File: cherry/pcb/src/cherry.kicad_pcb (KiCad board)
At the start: 4 copper layers, 61.2 x 26.1 mm, 73 parts, among them J1 USB4085-GF-A, J2 PinHeader_1x24, J3 PinHeader_1x24, J4 PinHeader_1x06, J5 PinHeader_1x06, J6 PinHeader_1x06, SW1 RESET, SW2 USER, U1 FT2232HL, U2 W25Q32JVSSIM, U3 ICE40LP8K-CM81, U4 TPS62A02, U5 TPS62A02, X1 ASE-12.000MHZ-LR-T

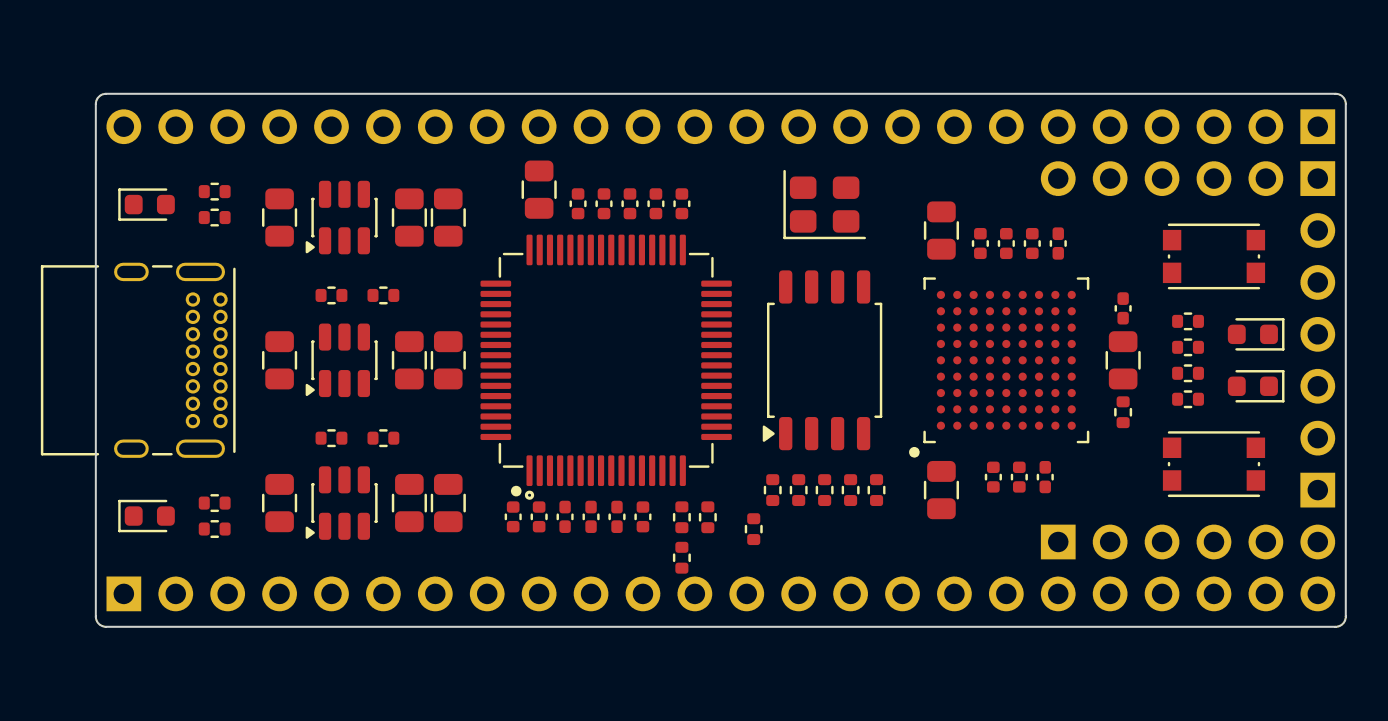
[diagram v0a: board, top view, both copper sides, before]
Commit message: wip
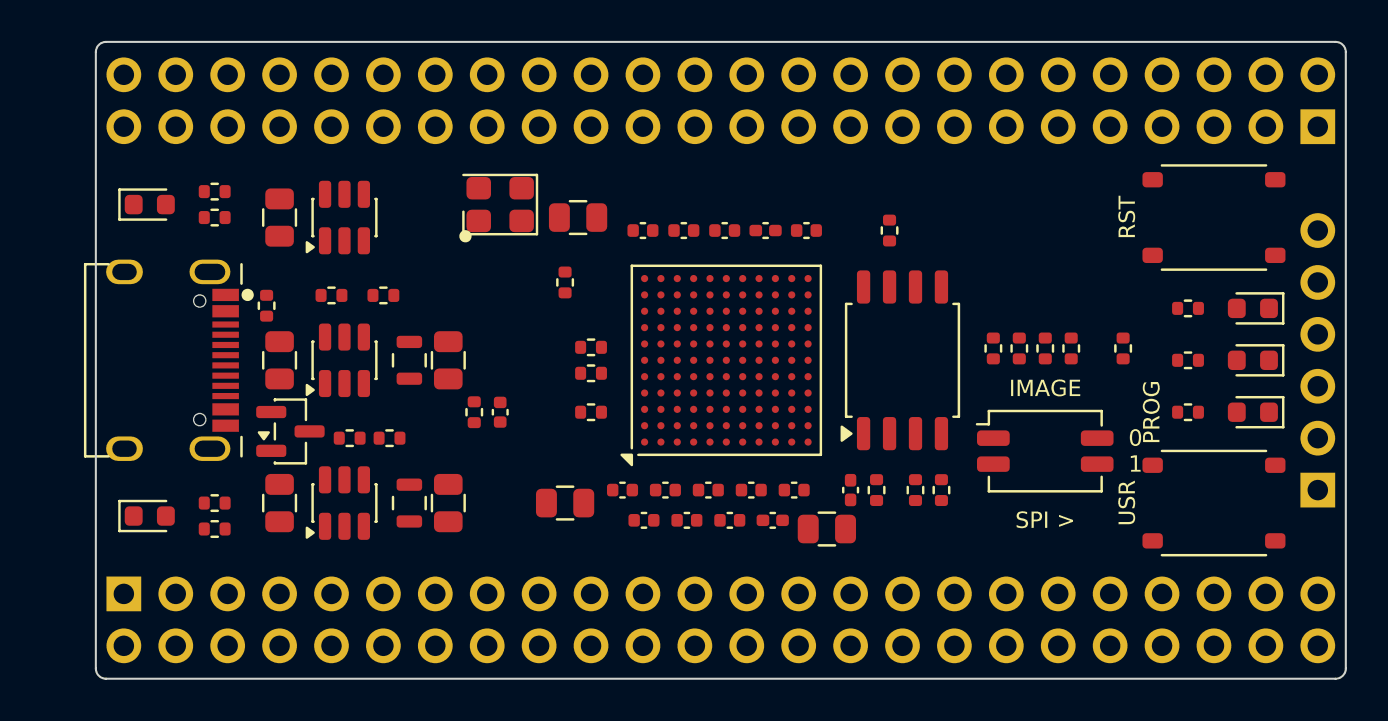
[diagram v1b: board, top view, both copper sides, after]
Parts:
- removed C12, C13, C14, C15: 100nF, Cherry:C_0402_1005Metric
- removed C26, C5: 10uF, Cherry:C_0805_2012Metric
- removed FB2: BLM21AG601SH1D, Cherry:L_0805_2012Metric
- removed J4, J6: PinHeader_1x06, Cherry:PinHeader_1x06_P2.54mm
- removed R18: 1k, Cherry:R_0402_1005Metric
- removed R7: 12k, Cherry:R_0402_1005Metric
- removed U1: FT2232HL, Cherry:LQFP-64_10x10mm_P0.5mm
- added C29: 100nF, Cherry:C_0402_1005Metric, F.Cu at (120.0, 92.7)
- added D6: LED_AMBER_0603, Cherry:LED_0603_1608Metric, F.Cu at (156.8, 92.7)
- added Q1: BSS138, Package_TO_SOT_SMD:SOT-23, F.Cu at (109.8, 93.7)
- added R23: 10k, Cherry:R_0402_1005Metric, F.Cu at (146.7, 89.6)
- added R24: 10k, Cherry:R_0402_1005Metric, F.Cu at (148.0, 89.6)
- added R25: 1k, Cherry:R_0402_1005Metric, F.Cu at (144.1, 89.6)
- added R26: 1k, Cherry:R_0402_1005Metric, F.Cu at (145.4, 89.6)
- added R27: 10k, Cherry:R_0402_1005Metric, F.Cu at (150.5, 89.6)
- added R29: 1k, Cherry:R_0402_1005Metric, F.Cu at (153.7, 92.7)
- added SW3: USER, Cherry:SW_Tactile_XKB_TS-1187A, F.Cu at (154.9, 97.2)
- D1: value PWR -> KT-0603R
- D2: value CFG -> KT-0603R
- D3: value USER0 -> KT-0603R
- D4: value USER1 -> KT-0603R
- FB1: value BLM21AG601SH1D -> GZ2012D601TF
- J1: value USB4085-GF-A -> TYPE-C-31-M-12; footprint Cherry:USB_C_Receptacle_GCT_USB4085 -> Cherry:USB_C_Receptacle_Hroparts_TYPE-C-31-M-12
- J2, J3: value PinHeader_1x24 -> PinHeader_2x24_Duplicate; footprint Cherry:PinHeader_1x24_P2.54mm -> Cherry:PinHeader_2x24_P2.54mm_Duplicate
- J5: value PinHeader_1x06 -> SPI PROGRAM
- L1, L2: value 1uH -> TFM201208ALD-1R0MTCA; footprint Cherry:L_0805_2012Metric -> Cherry:L_TDK_TFM201208ALD
- R14, R15: value 470 -> 68
- R16: value 470 -> 1.5k
- R17: value 470 -> 10k
- R9: value 10k -> 100k
- SW1: value RESET -> TS-1187A-B-A-B; footprint Cherry:SW_Push_1P1T_NO_CK_KMR2 -> Cherry:SW_Tactile_XKB_TS-1187A
- SW2: value USER -> IMAGE SELECT; footprint Cherry:SW_Push_1P1T_NO_CK_KMR2 -> Button_Switch_SMD:SW_DIP_SPSTx02_Slide_Copal_CHS-02A_W5.08mm_P1.27mm_JPin
- U2: value W25Q32JVSSIM -> W25Q32JVSSIQ
- U3: value ICE40LP8K-CM81 -> ICE40HX8K-BG121; footprint Cherry:BGA-81_9x9_8.0x8.0mm_P0.8mm -> Package_BGA:BGA-121_9.0x9.0mm_Layout11x11_P0.8mm_Ball0.4mm_Pad0.35mm_NSMD
- U4, U5: value TPS62A02 -> TPS62A02APDDCR
- X1: value ASE-12.000MHZ-LR-T -> OXETDLJANF-48.000000MHz; footprint Cherry:Oscillator_SMD_Abracon_ASE-4Pin_3.2x2.5mm -> Cherry:Oscillator_SMD_Taitien_OX_3.2x2.5mm
- moved R9 35.2 mm to (118.7, 92.7), turned to 90 degrees
- moved R12 26.2 mm to (108.6, 87.5)
- moved C6 18.4 mm to (123.2, 97.2), turned to 0 degrees
- moved C19 17.8 mm to (127.0, 83.8), turned to 0 degrees
- moved C7 17.8 mm to (123.8, 83.2), turned to 0 degrees
- moved C22 17.1 mm to (129.0, 83.8), turned to 0 degrees
- moved R11 16.8 mm to (139.1, 83.8), turned to 90 degrees
- moved C27 16.7 mm to (136.0, 98.4), turned to 0 degrees
- moved C28 16.0 mm to (137.2, 96.5)
- moved X1 15.9 mm to (120.0, 82.5)
- moved C25 15.6 mm to (134.4, 96.5), turned to 0 degrees
- moved C10 15.5 mm to (127.0, 98.0), turned to 0 degrees
- moved R17 15.3 mm to (123.2, 86.4)
- moved C11 14.6 mm to (128.1, 96.5), turned to 0 degrees
- moved R14 14.5 mm to (124.5, 89.5), turned to 0 degrees
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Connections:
- D2 pad 1: GND -> /CFG_LED_K
- D5 pad 4: /USB_DP -> /USB_DP_ESD
- D5 pad 6: /USB_DM -> /USB_DM_ESD
- J3 pad 10: /GPIO_28 -> unconnected-(J3-Pad10)
- J3 pad 13: /GPIO_31 -> unconnected-(J3-Pad13)
- J3 pad 9: /GPIO_27 -> unconnected-(J3-Pad9)
- J5 pad 1: /GPIO_43 -> GND
- J5 pad 2: /GPIO_44 -> /CRESET_B
- J5 pad 3: /GPIO_45 -> /QSPI_CS_B
- J5 pad 4: /GPIO_46 -> /QSPI_SCK
- J5 pad 5: /GPIO_47 -> /QSPI_IO0
- J5 pad 6: /GPIO_48 -> /QSPI_IO1
- R10 pad 2: /SPI_SS -> /QSPI_CS_B
- R11 pad 2: /BTN -> /QSPI_IO3
- R14 pad 1: /FT_SCK -> /USB_DP_ESD
- R14 pad 2: /SPI_SCK -> /USB_DP_FPGA
- R15 pad 1: /FT_MOSI -> /USB_DM_ESD
- R15 pad 2: /SPI_MOSI -> /USB_DM_FPGA
- R16 pad 1: /FT_MISO -> /USB_PULLUP
- R16 pad 2: /SPI_MISO -> /USB_DP_FPGA
- R17 pad 1: /FT_SS -> /CRESET_B
- R17 pad 2: /SPI_SS -> +3V3
- R20 pad 1: /CDONE -> +3V3
- R8 pad 2: Net-(U1-~{RESET}) -> /QSPI_IO2
- R9 pad 1: +3V3 -> +5V
- R9 pad 2: /CRESET_B -> /PWR_EN
- SW1 pad 1: /CRESET_B -> /PWR_EN
- SW2 pad 1: /BTN -> Net-(R25-Pad2)
- SW2 pad 2: GND -> Net-(R26-Pad2)
- U2 pad 1: /SPI_SS -> /QSPI_CS_B
- U2 pad 2: /SPI_MISO -> /QSPI_IO1
- U2 pad 3: +3V3 -> /QSPI_IO2
- U2 pad 5: /SPI_MOSI -> /QSPI_IO0
- U2 pad 6: /SPI_SCK -> /QSPI_SCK
- U2 pad 7: +3V3 -> /QSPI_IO3
- U3 pad A3: /GPIO_31 -> /USB_PULLUP
- U3 pad A4: /GPIO_27 -> /USB_DM_FPGA
- U3 pad A5: +3V3 -> /GPIO_12
- U3 pad A9: /GPIO_46 -> unconnected-(U3-IOT_178-PadA9)
- U3 pad B4: /GPIO_28 -> /USB_DP_FPGA
- U3 pad B9: /GPIO_50 -> unconnected-(U3-IOT_174-PadB9)
- U3 pad C4: /BTN -> /USER_BTN
- U3 pad C5: /GPIO_26 -> /GNDPLL
- U3 pad C6: +3V3 -> /VCCPLL
- U3 pad C7: unconnected-(U3-VPP_FAST-PadC7) -> /GPIO_26
- U3 pad C8: +3V3 -> /GPIO_30
- U3 pad C9: /GPIO_53 -> unconnected-(U3-IOT_172-PadC9)
- U3 pad D6: /GPIO_45 -> +3V3
- U3 pad D7: /GPIO_47 -> unconnected-(U3-IOT_181-PadD7)
- U3 pad D8: /GPIO_52 -> +1V2
- U3 pad D9: /GPIO_49 -> unconnected-(U3-IOR_147-PadD9)
- U3 pad E4: /GPIO_12 -> +3V3
- U3 pad E5: /GPIO_30 -> GND
- U3 pad E6: /CDONE -> GND
- U3 pad E7: /GPIO_48 -> GND
- U3 pad E8: /GPIO_51 -> unconnected-(U3-IOR_146-PadE8)
- U3 pad E9: +1V2 -> unconnected-(U3-IOR_144-PadE9)
- U3 pad F2: +1V2 -> unconnected-(U3-IOL_12B-PadF2)
- U3 pad F4: GND -> unconnected-(U3-IOL_13A-PadF4)
- U3 pad F7: /SPI_SS -> GND
- U3 pad F8: /GPIO_43 -> +3V3
- U3 pad F9: GND -> unconnected-(U3-IOR_137-PadF9)
- U3 pad G4: /CLK_12M -> +3V3
- U3 pad G5: /GPIO_40 -> GND
- U3 pad G6: /SPI_MOSI -> GND
- U3 pad G7: /SPI_SCK -> GND
- U3 pad G8: /GPIO_44 -> unconnected-(U3-IOR_118-PadG8)
- U3 pad G9: /GPIO_42 -> unconnected-(U3-IOR_128-PadG9)
- U3 pad H3: +3V3 -> unconnected-(U3-IOL_17B-PadH3)
- U3 pad H4: /GPIO_39 -> +1V2
- U3 pad H5: /GPIO_41 -> GND
- U3 pad H6: /CRESET_B -> +3V3
- U3 pad H7: /SPI_MISO -> unconnected-(U3-IOB_87-PadH7)
- U3 pad H8: +3V3 -> +1V2
- U3 pad H9: /UART_RX -> /CBSEL1
- U3 pad J2: /GPIO_37 -> unconnected-(U3-IOL_25B-PadJ2)
- U3 pad J3: /GPIO_38 -> /LED1
- U3 pad J5: +3V3 -> unconnected-(U3-IOB_78-PadJ5)
- U3 pad J6: /GNDPLL -> /VCCPLL
- U3 pad J7: /VCCPLL -> unconnected-(U3-IOB_86-PadJ7)
- U3 pad J8: /UART_TX -> /QSPI_IO3
- U3 pad J9: /LED1 -> /QSPI_IO1
- U4 pad 1: +5V -> /PWR_EN
- U5 pad 1: +5V -> /PWR_EN
- X1 pad 3: /CLK_12M -> /CLK_48M
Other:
- board size 61.2 x 26.1 mm -> 61.2 x 31.2 mm
- board text added: "0"
- board text added: "1"
- board text added: "IMAGE"
- board text added: "PROG"
- board text added: "RST"
- board text added: "SPI >"
- board text added: "USR"
